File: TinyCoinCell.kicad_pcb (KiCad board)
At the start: 4 copper layers, 23.8 x 24 mm, 51 parts, among them SW1 SW_Push, U1 nRF54L15-QFAA, U2 ADXL367, U8 nPM2100-QEXX, X1 32MHz, X2 32.768kHz

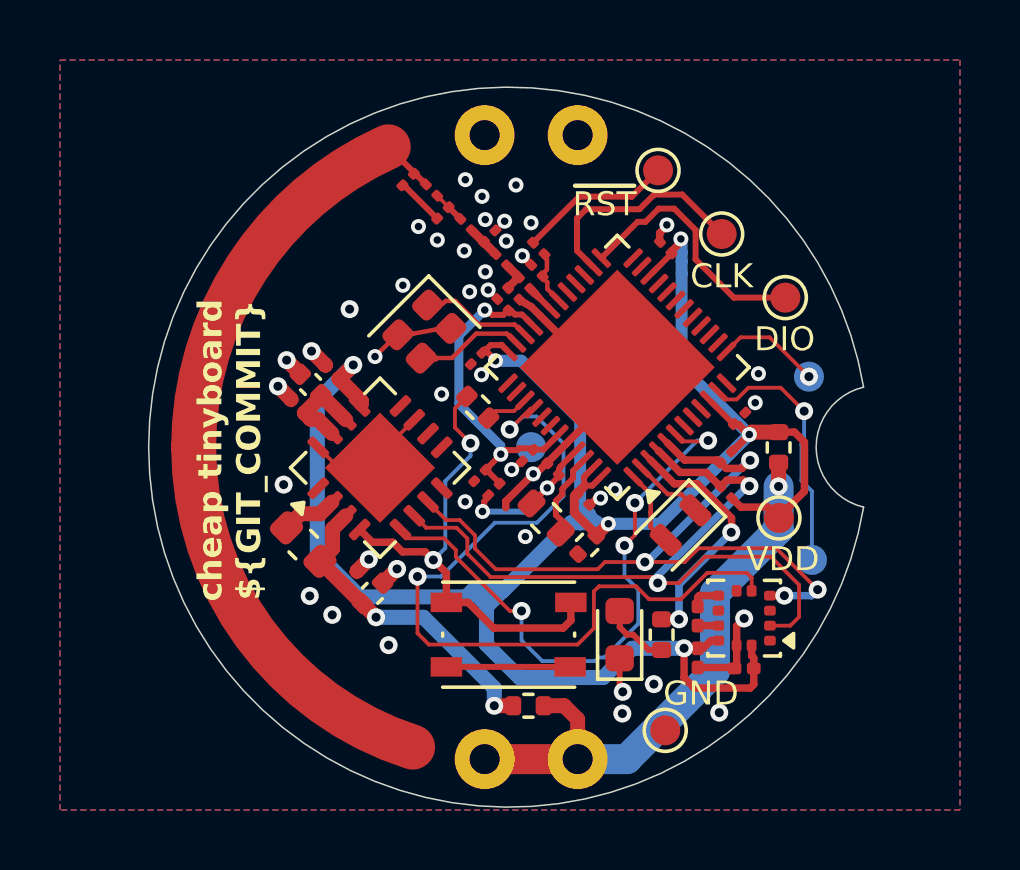
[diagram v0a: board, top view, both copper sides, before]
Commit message: Updated PCB
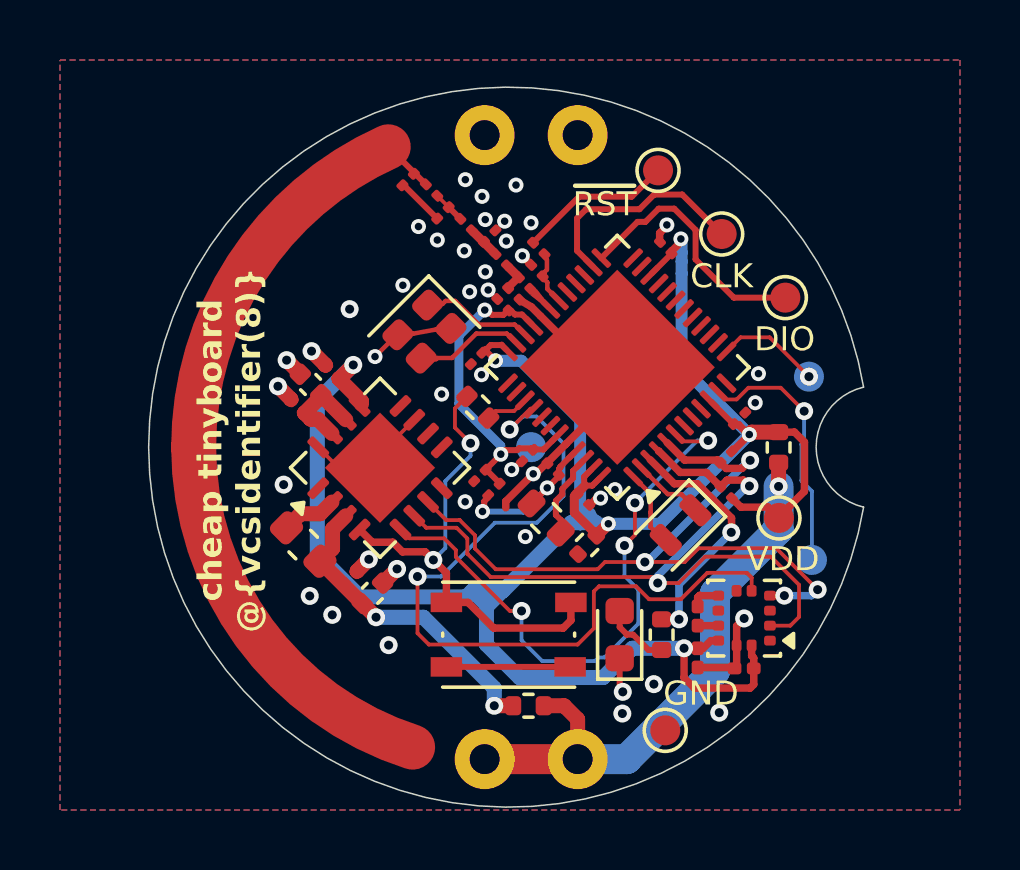
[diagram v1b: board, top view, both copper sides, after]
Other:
- board text added: "cheap tinyboard @{vcsidentifier(8)}"
- board text removed: "cheap tinyboard ${GIT_COMMIT}"
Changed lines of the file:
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@@
 		)
 	)
-	(gr_text "cheap tinyboard \n${GIT_COMMIT}\n"
+	(gr_text "cheap tinyboard \n@{vcsidentifier(8)}\n"
 		(at 134.49516 112.19522 90)
 		(layer "F.SilkS")
